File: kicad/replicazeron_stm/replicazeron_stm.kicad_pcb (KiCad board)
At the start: 2 copper layers, 41 parts, among them J10 Conn_01x04_Pin, J1_Col1 Conn_01x06_Pin, J2_Thumb1 Conn_01x06_Pin, J3_Index1 Conn_01x06_Pin, J4_Mid1 Conn_01x06_Pin, J5_Ring1 Conn_01x06_Pin, J6_Pinky1 Conn_01x06_Pin, J7_Stick1 Conn_01x02_Pin, J8_LED1 Conn_01x02_Pin, J9 Conn_01x03_Pin, U2 YAAJ_BluePill

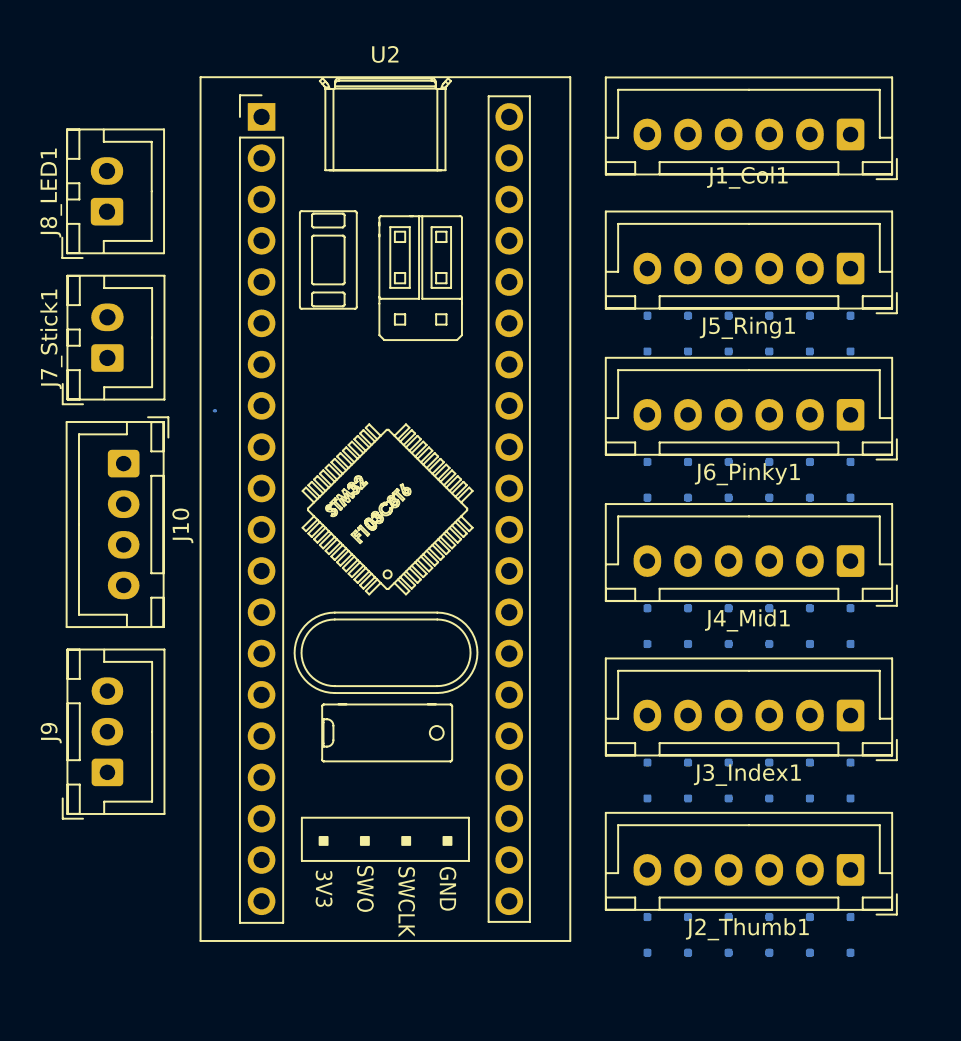
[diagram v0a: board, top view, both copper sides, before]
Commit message: Routing PCB Version A
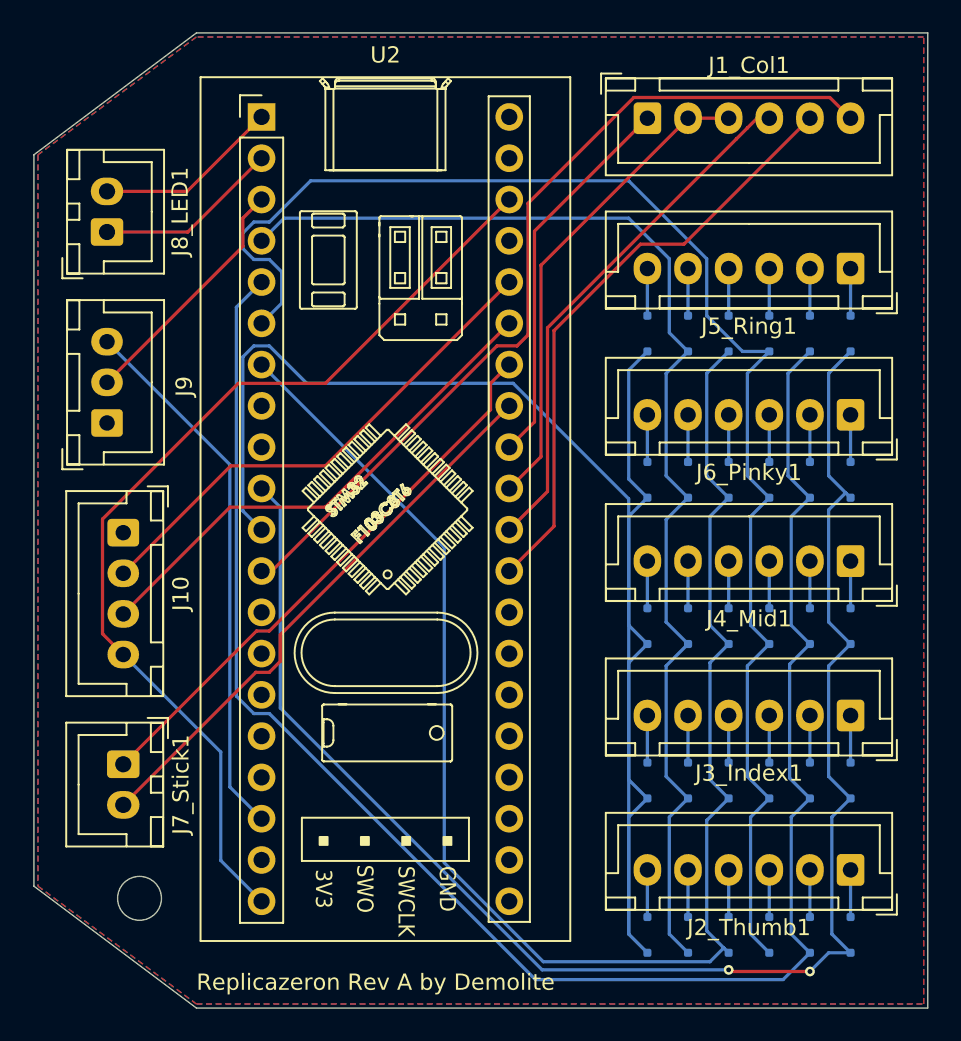
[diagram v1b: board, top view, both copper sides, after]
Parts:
- added REF**: MountingHole_2.7mm_M2.5, MountingHole:MountingHole_2.7mm_M2.5, F.Cu at (74.0, 90.8)
- moved J7_Stick1 25.0 mm to (73.0, 82.5), turned to -90 degrees
- moved J9 21.5 mm to (72.0, 61.5)
- moved J1_Col1 12.5 mm to (105.2, 42.8), turned to 0 degrees
- moved J10 4.25 mm to (73.0, 68.2)
- moved J8_LED1 1.25 mm to (72.0, 49.8)
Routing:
- net row_1: track 0.00 -> 110.4 mm
- net row_5: track 0.00 -> 106.6 mm
- net row_0: track 0.00 -> 97.7 mm, vias 0 -> 2
- net row_3: track 0.07 -> 96.5 mm
- net row_2: track 0.00 -> 88.9 mm
- net row_4: track 0.00 -> 74.2 mm
- net +3.3V: track 0.00 -> 60.7 mm
- net col_4: track 0.00 -> 53.6 mm
- net col_3: track 0.00 -> 37.1 mm
- net axis_0: track 0.00 -> 34.9 mm
- net axis_1: track 0.00 -> 34.9 mm
- net +5V: track 0.00 -> 33.3 mm
- net col_2: track 0.00 -> 32.4 mm
- net i2c_sda: track 0.00 -> 31.2 mm
- net i2c_scl: track 0.00 -> 31.2 mm
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- added copper zone on F.Cu, net +5V
- added copper zone on B.Cu, net GND
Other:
- board outline added: 55 x 60 mm
- board text added: "Replicazeron Rev A by Demolite"
